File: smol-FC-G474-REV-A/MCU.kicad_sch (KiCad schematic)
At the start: 19 parts, among them J1 USB-C-16P, U1 STM32G474RETx, U2 USBLC6-2P6, Y1 8MHz

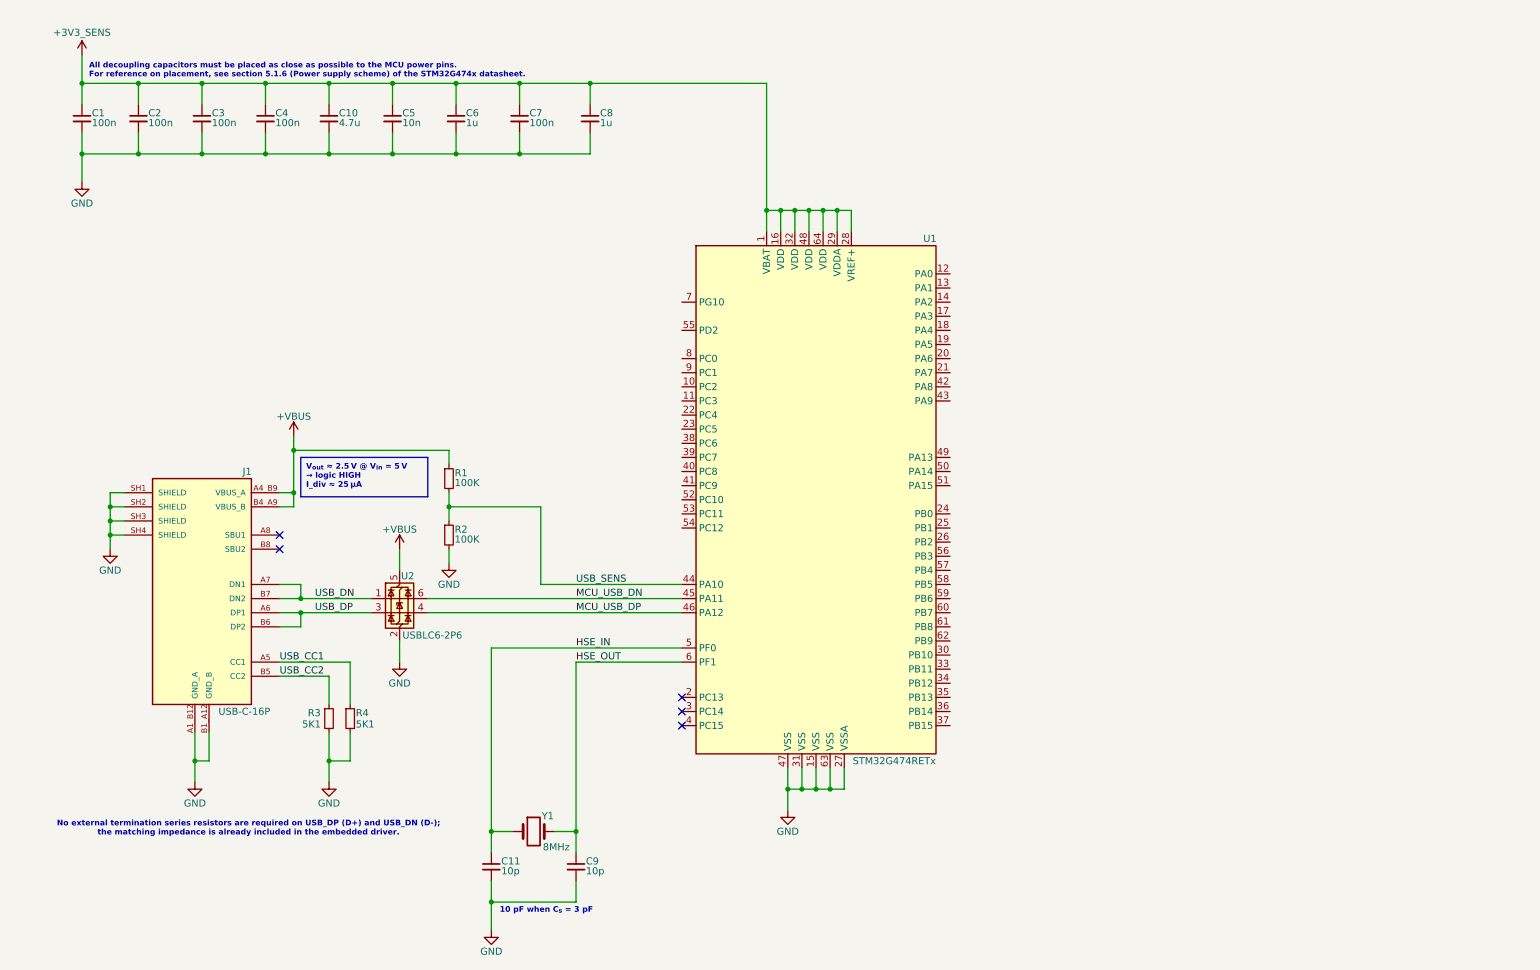
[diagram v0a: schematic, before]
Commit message: Schematic update
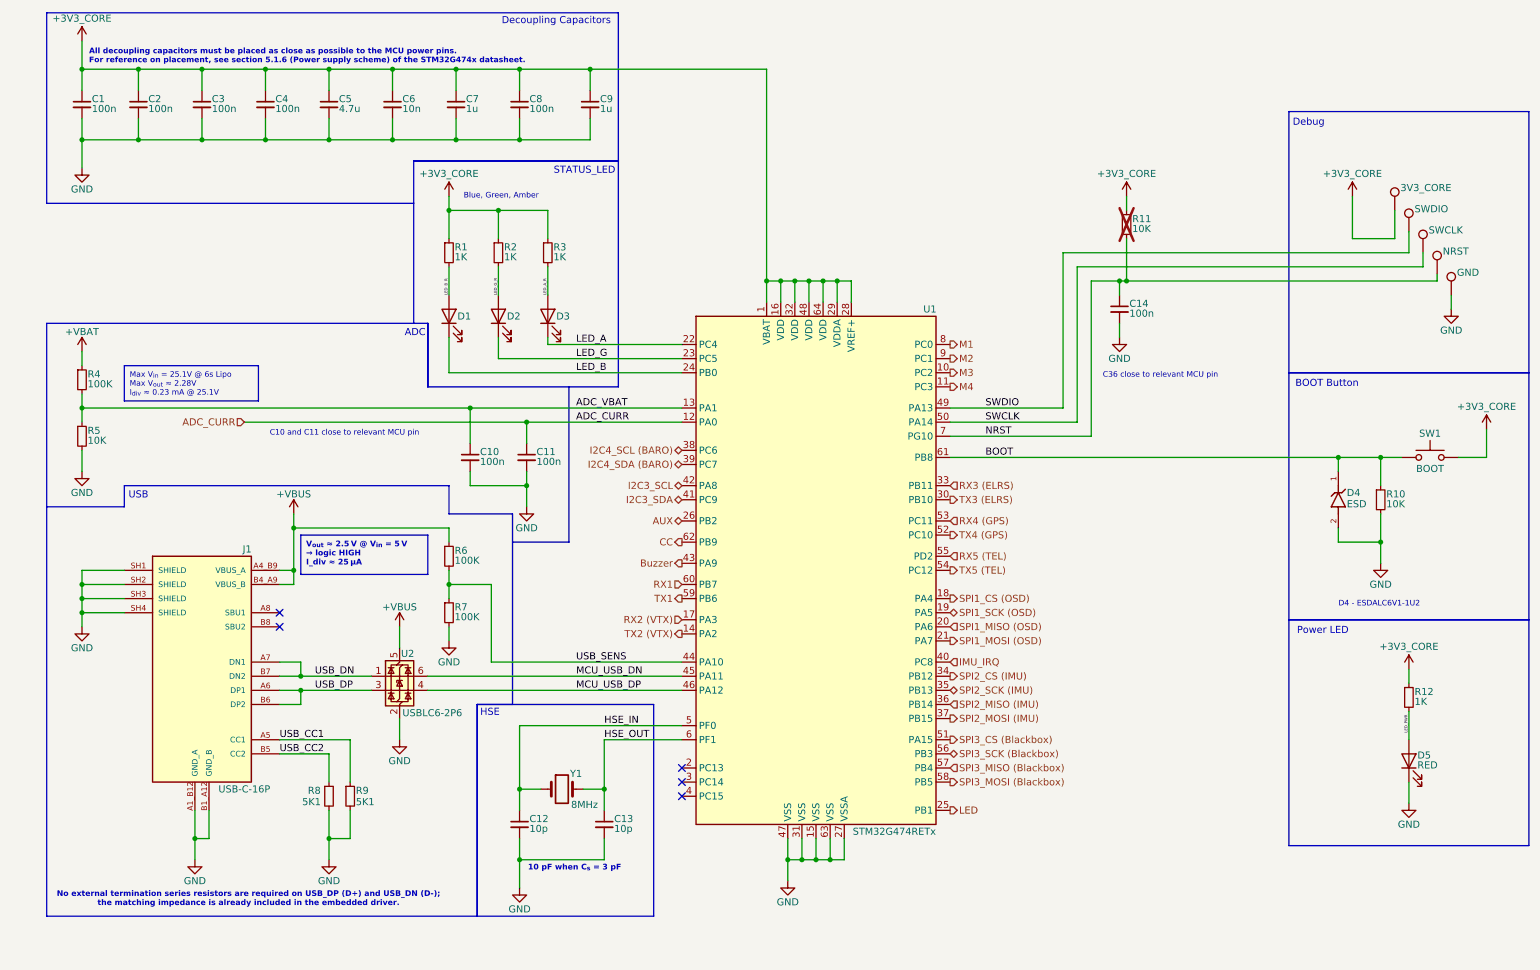
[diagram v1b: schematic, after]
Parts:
- added 3V3_CORE, GND, NRST, SWCLK, SWDIO: TestPoint, symbol Connector:TestPoint
- added C10, C11, C14: 100n, symbol Device:C_Small
- added D1, D2, D3: LED, symbol Device:LED
- added D4: ESD, ESDALC6V1-1U2:DIODE_ESDALC6V1-1U2, symbol ESDALC6V1-1U2:ESDALC6V1-1U2
- added D5: RED, symbol Device:LED
- added R1, R12, R2, R3: 1K, symbol Device:R_Small
- added R10, R11, R5: 10K, symbol Device:R_Small
- added R4: 100K, symbol Device:R_Small
- added SW1: BOOT, symbol Switch:SW_Push
- renumbered C11 to C12, C9 to C13, C10 to C5, C5 to C6, C6 to C7, C7 to C8, C8 to C9, R1 to R6, R2 to R7, R3 to R8, R4 to R9
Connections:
- net GND: now also C10.2, C11.2, C14.2, D4.2, D5.1 (K), GND.1, R10.2, R5.2
- net M3: now reaches U1.10 (PC2)
- net M4: now reaches U1.11 (PC3)
- net ADC_CURR: now reaches U1.12 (PA0)
- net ADC_CURR: now also C11.1
- net ADC_VBAT: now reaches U1.13 (PA1)
- net ADC_VBAT: now also C10.1, R4.2, R5.1
- net TX2 (VTX): now reaches U1.14 (PA2)
- net RX2 (VTX): now reaches U1.17 (PA3)
- net SPI1_CS (OSD): now reaches U1.18 (PA4)
- net SPI1_SCK (OSD): now reaches U1.19 (PA5)
- net SPI1_MISO (OSD): now reaches U1.20 (PA6)
- net SPI1_MOSI (OSD): now reaches U1.21 (PA7)
- net LED_A: now reaches U1.22 (PC4)
- net LED_A: now also D3.1 (K)
- net LED_G: now reaches U1.23 (PC5)
- net LED_G: now also D2.1 (K)
- net LED_B: now reaches U1.24 (PB0)
- net LED_B: now also D1.1 (K)
- net LED: now reaches U1.25 (PB1)
- net AUX: now reaches U1.26 (PB2)
- net TX3 (ELRS): now reaches U1.30 (PB10)
- net RX3 (ELRS): now reaches U1.33 (PB11)
- net SPI2_CS (IMU): now reaches U1.34 (PB12)
- net SPI2_SCK (IMU): now reaches U1.35 (PB13)
- net SPI2_MISO (IMU): now reaches U1.36 (PB14)
- net SPI2_MOSI (IMU): now reaches U1.37 (PB15)
- net I2C4_SCL (BARO): now reaches U1.38 (PC6)
- net I2C4_SDA (BARO): now reaches U1.39 (PC7)
- net IMU_IRQ: now reaches U1.40 (PC8)
- net I2C3_SDA: now reaches U1.41 (PC9)
- net I2C3_SCL: now reaches U1.42 (PA8)
- net Buzzer: now reaches U1.43 (PA9)
- net SWDIO: now reaches U1.49 (PA13)
- net SWDIO: now also SWDIO.1
- net SWCLK: now reaches U1.50 (PA14)
- net SWCLK: now also SWCLK.1
- net SPI3_CS (Blackbox): now reaches U1.51 (PA15)
- net TX4 (GPS): now reaches U1.52 (PC10)
- net RX4 (GPS): now reaches U1.53 (PC11)
- net TX5 (TEL): now reaches U1.54 (PC12)
- net RX5 (TEL): now reaches U1.55 (PD2)
- net SPI3_SCK (Blackbox): now reaches U1.56 (PB3)
- net SPI3_MISO (Blackbox): now reaches U1.57 (PB4)
- net SPI3_MOSI (Blackbox): now reaches U1.58 (PB5)
- net TX1: now reaches U1.59 (PB6)
- net RX1: now reaches U1.60 (PB7)
- net BOOT: now reaches U1.61 (PB8)
- net BOOT: now also D4.1, R10.1, SW1.1
- net CC: now reaches U1.62 (PB9)
- net NRST: now reaches U1.7 (PG10)
- net NRST: now also C14.1, NRST.1, R11.2
- net M1: now reaches U1.8 (PC0)
- net M2: now reaches U1.9 (PC1)
- net +3V3_SENS renamed +3V3_CORE
- net +3V3_CORE: now also 3V3_CORE.1, R1.1, R11.1, R12.1, R2.1, R3.1, SW1.2
- new net +VBAT: R4.1
- new net LED_A_R: D3.2 (A), R3.2
- new net LED_B_R: D1.2 (A), R1.2
- new net LED_G_R: D2.2 (A), R2.2
- new net LED_PWR: D5.2 (A), R12.2
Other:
- note added: "ADC"
- note added: "BOOT Button"
- note added: "Blue, Green, Amber"
- note added: "C10 and C11 close to relevant MCU pin"
- note added: "C36 close to relevant MCU pin"
- note added: "D4 - ESDALC6V1-1U2"
- note added: "Debug"
- note added: "Decoupling Capacitors"
- note added: "HSE"
- note added: "Power LED"
- note added: "STATUS_LED"
- note added: "USB"
- moved on the sheet: C1, C12, C13, C2, C3, C4, C5, C6, C7, C8, C9, J1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
